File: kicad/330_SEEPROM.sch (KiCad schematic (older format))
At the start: 5 parts, among them J330 Conn_02x04_Top_Bottom, U330 25LCxxx, U331 74LS126

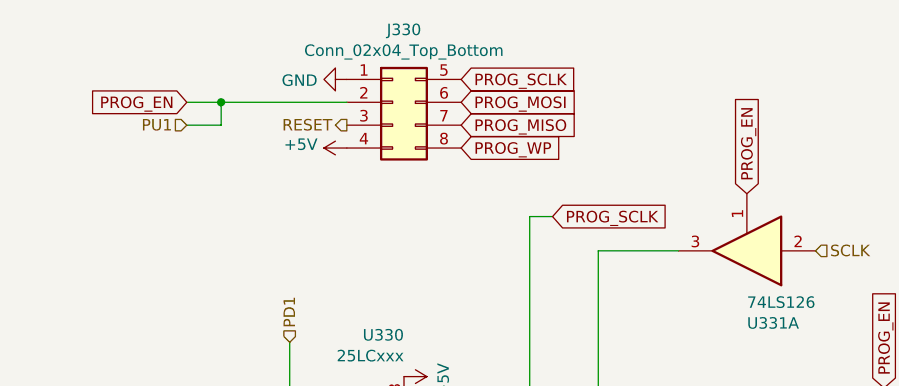
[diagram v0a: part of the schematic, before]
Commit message: redid layout
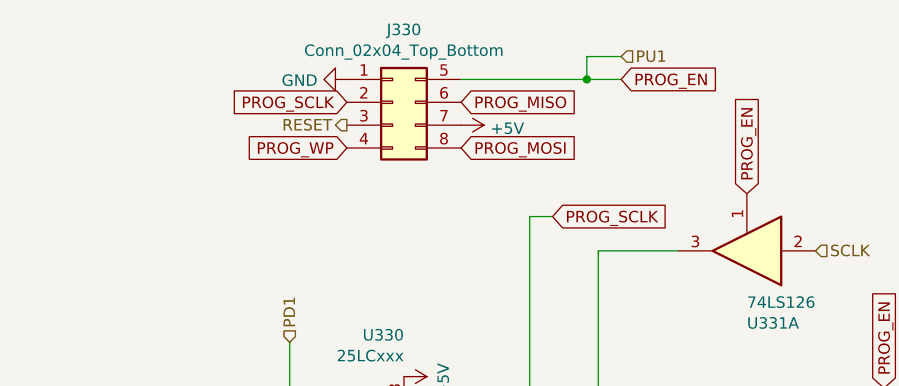
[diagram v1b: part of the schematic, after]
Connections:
- net +5V: now also J330.7 (Pin_7); no longer J330.4 (Pin_4)
- net PROG_EN: now also J330.5 (Pin_5); no longer J330.2 (Pin_2)
- net PROG_MISO: now also J330.6 (Pin_6); no longer J330.7 (Pin_7)
- net PROG_MOSI: now also J330.8 (Pin_8); no longer J330.6 (Pin_6)
- net PROG_SCLK: now also J330.2 (Pin_2); no longer J330.5 (Pin_5)
- net PROG_WP: now also J330.4 (Pin_4); no longer J330.8 (Pin_8)
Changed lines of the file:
@@
 Text GLabel 5550 2950 2    50   Input ~ 0
 PROG_SCLK
-Text GLabel 3950 2450 0    50   Input ~ 0
-PROG_EN
 Text GLabel 4300 3850 0    50   Input ~ 0
 PROG_WP
-Wire Wire Line
-	3950 2450 4100 2450
-Wire Wire Line
-	3950 2550 4100 2550
-Wire Wire Line
-	4100 2550 4100 2450
 $Comp
 L 74xx:74LS126 U?
@@
 Wire Wire Line
 	4400 3850 4500 3850
-Text GLabel 5150 2650 2    50   Input ~ 0
+Text GLabel 4650 2650 0    50   Input ~ 0
 PROG_WP
 Text Notes 7200 5650 0    50   ~ 0
@@
 Text HLabel 6700 3100 2    50   Input ~ 0
 SCLK
-Text HLabel 3950 2550 0    50   Input ~ 0
-PU1
 Text HLabel 4500 3950 0    50   Input ~ 0
 PU2
@@
 Wire Wire Line
 	6700 4350 6950 4350
-Text GLabel 5150 2350 2    50   Input ~ 0
+Text GLabel 4650 2450 0    50   Input ~ 0
 PROG_SCLK
+Text GLabel 5150 2650 2    50   Input ~ 0
+PROG_MOSI
 Text GLabel 5150 2450 2    50   Input ~ 0
-PROG_MOSI
-Text GLabel 5150 2550 2    50   Input ~ 0
 PROG_MISO
-$Comp
-L power:+5V #PWR0156
-U 1 1 619F2BF3
-P 4650 2650
-F 0 "#PWR0156" H 4650 2500 50  0001 C CNN
-F 1 "+5V" V 4665 2778 50  0000 L CNN
-F 2 "" H 4650 2650 50  0001 C CNN
-F 3 "" H 4650 2650 50  0001 C CNN
-	1    4650 2650
-	0    -1   -1   0
-$EndComp
-$Comp
-L power:GND #PWR0157
-U 1 1 619F365E
-P 4650 2350
-F 0 "#PWR0157" H 4650 2100 50  0001 C CNN
-F 1 "GND" V 4655 2222 50  0000 R CNN
-F 2 "" H 4650 2350 50  0001 C CNN
-F 3 "" H 4650 2350 50  0001 C CNN
-	1    4650 2350
-	0    1    1    0
-$EndComp
 $Comp
 L Device:C C?
@@
 Text Notes 7000 6650 0    50   ~ 10
 This page has been checked\n
-Connection ~ 4100 2450
-Wire Wire Line
-	4100 2450 4650 2450
-Text HLabel 4650 2550 0    50   Output ~ 0
-RESET
 Text HLabel 4400 3500 1    50   Input ~ 0
 PD1
 Text HLabel 4400 4400 3    50   Input ~ 0
 PD2
+Text HLabel 4650 2550 0    50   Output ~ 0
+RESET
+Wire Wire Line
+	5700 2350 5150 2350
+Connection ~ 5700 2350
+$Comp
+L power:GND #PWR0157
+U 1 1 619F365E
+P 4650 2350
+F 0 "#PWR0157" H 4650 2100 50  0001 C CNN
+F 1 "GND" V 4655 2222 50  0000 R CNN
+F 2 "" H 4650 2350 50  0001 C CNN
+F 3 "" H 4650 2350 50  0001 C CNN
+	1    4650 2350
+	0    1    1    0
+$EndComp
+$Comp
+L power:+5V #PWR0156
+U 1 1 619F2BF3
+P 5150 2550
+F 0 "#PWR0156" H 5150 2400 50  0001 C CNN
+F 1 "+5V" V 5165 2678 50  0000 L CNN
+F 2 "" H 5150 2550 50  0001 C CNN
+F 3 "" H 5150 2550 50  0001 C CNN
+	1    5150 2550
+	0    1    1    0
+$EndComp
+Text HLabel 5850 2250 2    50   Input ~ 0
+PU1
+Wire Wire Line
+	5700 2250 5700 2350
+Wire Wire Line
+	5850 2250 5700 2250
+Wire Wire Line
+	5850 2350 5700 2350
+Text GLabel 5850 2350 2    50   Input ~ 0
+PROG_EN
 $EndSCHEMATC
